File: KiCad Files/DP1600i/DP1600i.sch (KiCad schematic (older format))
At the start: 7 parts, among them J3 Conn_01x07, J4 Conn_01x08, J5 Conn_01x04, J6 Conn_01x02, J7 Conn_02x04_Odd_Even, J8 Conn_01x05, J9 Conn_01x08

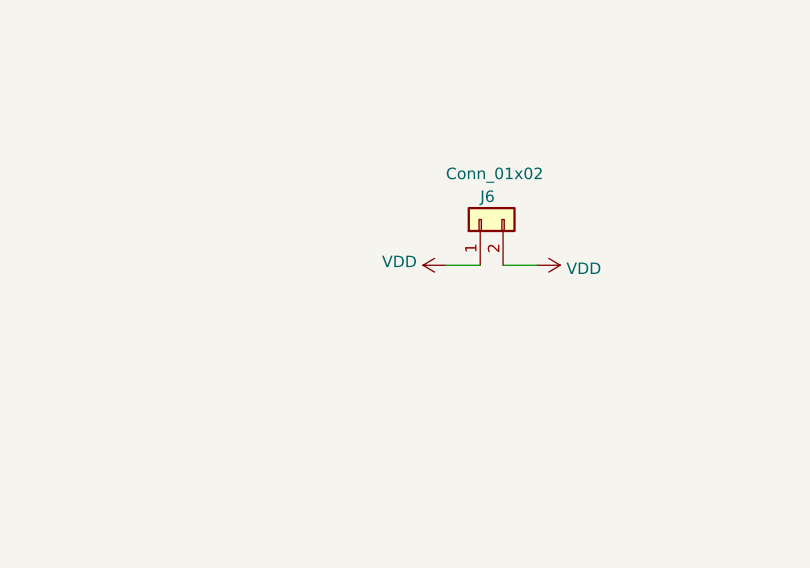
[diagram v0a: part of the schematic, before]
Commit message: Add files via upload
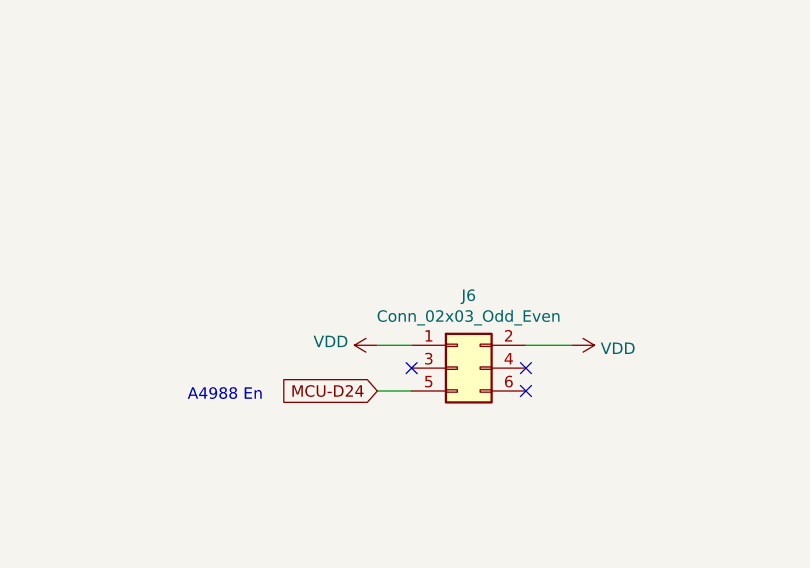
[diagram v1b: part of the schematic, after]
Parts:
- removed J6: Conn_01x02, Connector_PinHeader_2.54mm:PinHeader_1x02_P2.54mm_Vertical, symbol Connector_Generic:Conn_01x02
- added J6: Conn_02x03_Odd_Even, Connector_PinHeader_2.54mm:PinHeader_2x03_P2.54mm_Vertical, symbol Connector_Generic:Conn_02x03_Odd_Even
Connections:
- net VDD: now also J6.1 (Pin_1), J6.2 (Pin_2)
- new net MCU-D24: J6.5 (Pin_5)
- no-connect marks 1 -> 4
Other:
- note added: "A4988 En\n"
- note removed: "Spare\n"
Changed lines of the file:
@@
 L power:VDD #PWR02
 U 1 1 63826E84
-P 7900 2350
-F 0 "#PWR02" H 7900 2200 50  0001 C CNN
-F 1 "VDD" V 7915 2477 50  0000 L CNN
-F 2 "" H 7900 2350 50  0001 C CNN
-F 3 "" H 7900 2350 50  0001 C CNN
-	1    7900 2350
+P 7600 2700
+F 0 "#PWR02" H 7600 2550 50  0001 C CNN
+F 1 "VDD" V 7615 2827 50  0000 L CNN
+F 2 "" H 7600 2700 50  0001 C CNN
+F 3 "" H 7600 2700 50  0001 C CNN
+	1    7600 2700
 	0    -1   -1   0
 $EndComp
@@
 L power:VDD #PWR038
 U 1 1 63827375
-P 8300 2350
-F 0 "#PWR038" H 8300 2200 50  0001 C CNN
-F 1 "VDD" V 8315 2477 50  0000 L CNN
-F 2 "" H 8300 2350 50  0001 C CNN
-F 3 "" H 8300 2350 50  0001 C CNN
-	1    8300 2350
+P 8450 2700
+F 0 "#PWR038" H 8450 2550 50  0001 C CNN
+F 1 "VDD" V 8465 2827 50  0000 L CNN
+F 2 "" H 8450 2700 50  0001 C CNN
+F 3 "" H 8450 2700 50  0001 C CNN
+	1    8450 2700
 	0    1    1    0
 $EndComp
@@
 Text Notes 4000 2050 1    50   ~ 0
 Spare
-Text GLabel 4650 1400 3    50   Input ~ 0
-MCU-D0
+Text GLabel 7600 2900 0    50   Input ~ 0
+MCU-D24
 Text GLabel 4550 1400 3    50   Input ~ 0
 MCU-D1
-Text Notes 4700 2050 1    50   ~ 0
-Spare\n
+Text Notes 7100 2950 2    50   ~ 0
+A4988 En\n
 Text Notes 4600 2050 1    50   ~ 0
 Spare
@@
 Text Notes 4400 2050 1    50   ~ 0
 Spare
-$Comp
-L Connector_Generic:Conn_01x02 J6
-U 1 1 6390E746
-P 8050 2150
-F 0 "J6" V 8150 2150 50  0000 R CNN
-F 1 "Conn_01x02" V 8250 2300 50  0000 R CNN
-F 2 "Connector_PinHeader_2.54mm:PinHeader_1x02_P2.54mm_Vertical" H 8050 2150 50  0001 C CNN
-F 3 "~" H 8050 2150 50  0001 C CNN
-	1    8050 2150
-	0    -1   -1   0
-$EndComp
 $Comp
 L Connector_Generic:Conn_01x04 J5
@@
 $EndComp
 Wire Wire Line
-	8150 2350 8300 2350
-Wire Wire Line
-	7900 2350 8050 2350
-Wire Wire Line
 	8650 3950 8300 3950
 Wire Wire Line
@@
 	1    0    0    -1
 $EndComp
+$Comp
+L Connector_Generic:Conn_02x03_Odd_Even J6
+U 1 1 6394E4BE
+P 7950 2800
+F 0 "J6" H 8000 3117 50  0000 C CNN
+F 1 "Conn_02x03_Odd_Even" H 8000 3026 50  0000 C CNN
+F 2 "Connector_PinHeader_2.54mm:PinHeader_2x03_P2.54mm_Vertical" H 7950 2800 50  0001 C CNN
+F 3 "~" H 7950 2800 50  0001 C CNN
+	1    7950 2800
+	1    0    0    -1
+$EndComp
+Wire Wire Line
+	7750 2700 7600 2700
+Wire Wire Line
+	7600 2900 7750 2900
+Wire Wire Line
+	8450 2700 8250 2700
+Text GLabel 4650 1400 3    50   Input ~ 0
+MCU-D0
+Text Notes 4700 2050 1    50   ~ 0
+Spare
+NoConn ~ 7750 2800
+NoConn ~ 8250 2800
+NoConn ~ 8250 2900
 $EndSCHEMATC
